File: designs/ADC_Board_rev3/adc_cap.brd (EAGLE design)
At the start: 100 x 80 mm, 35 parts, among them Q1 BSS84, Q2 BSS84, Q3 BSS84, Q4 BSS84

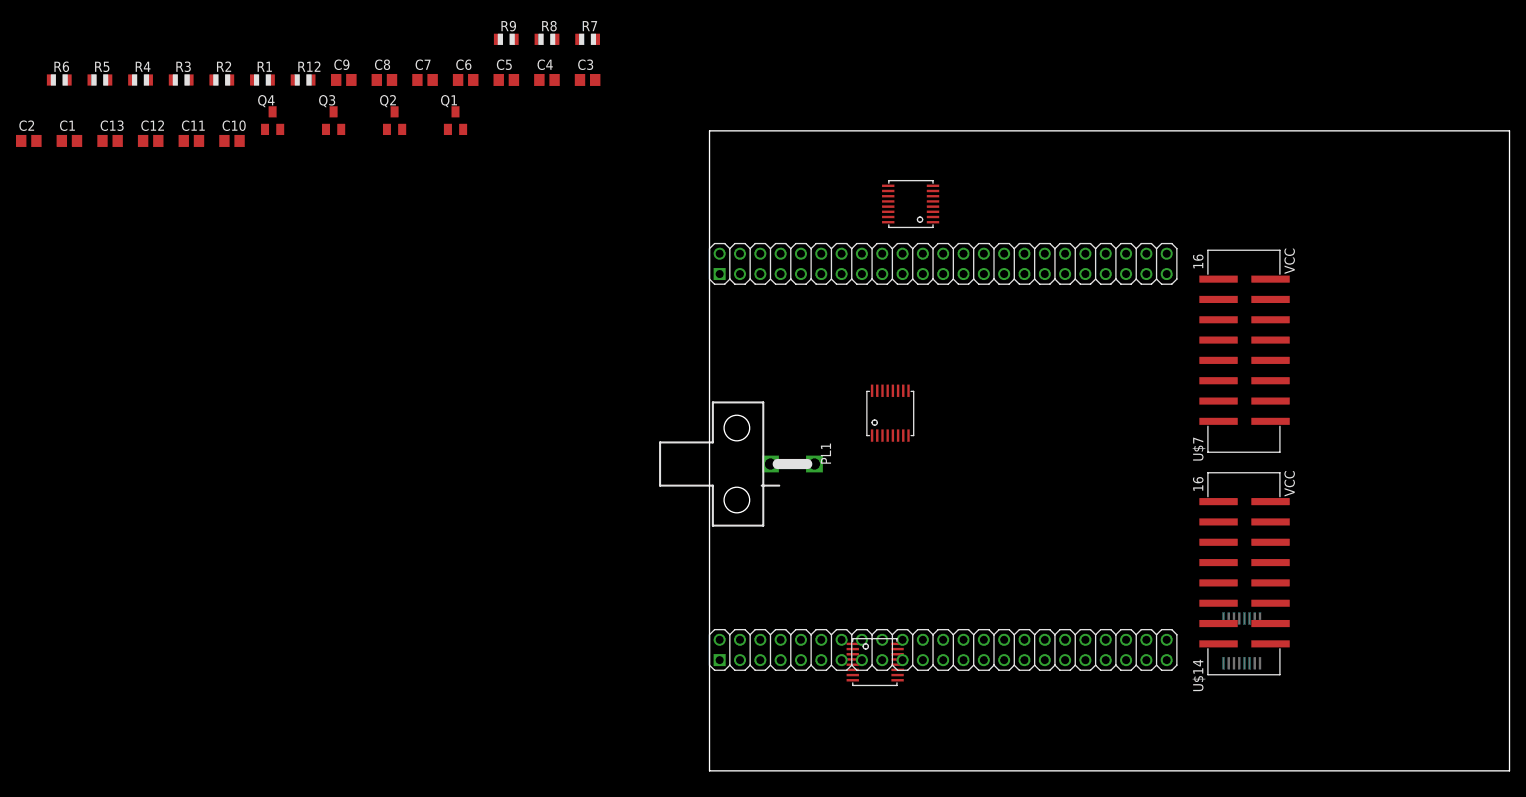
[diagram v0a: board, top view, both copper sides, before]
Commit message: Update on adc rev 3
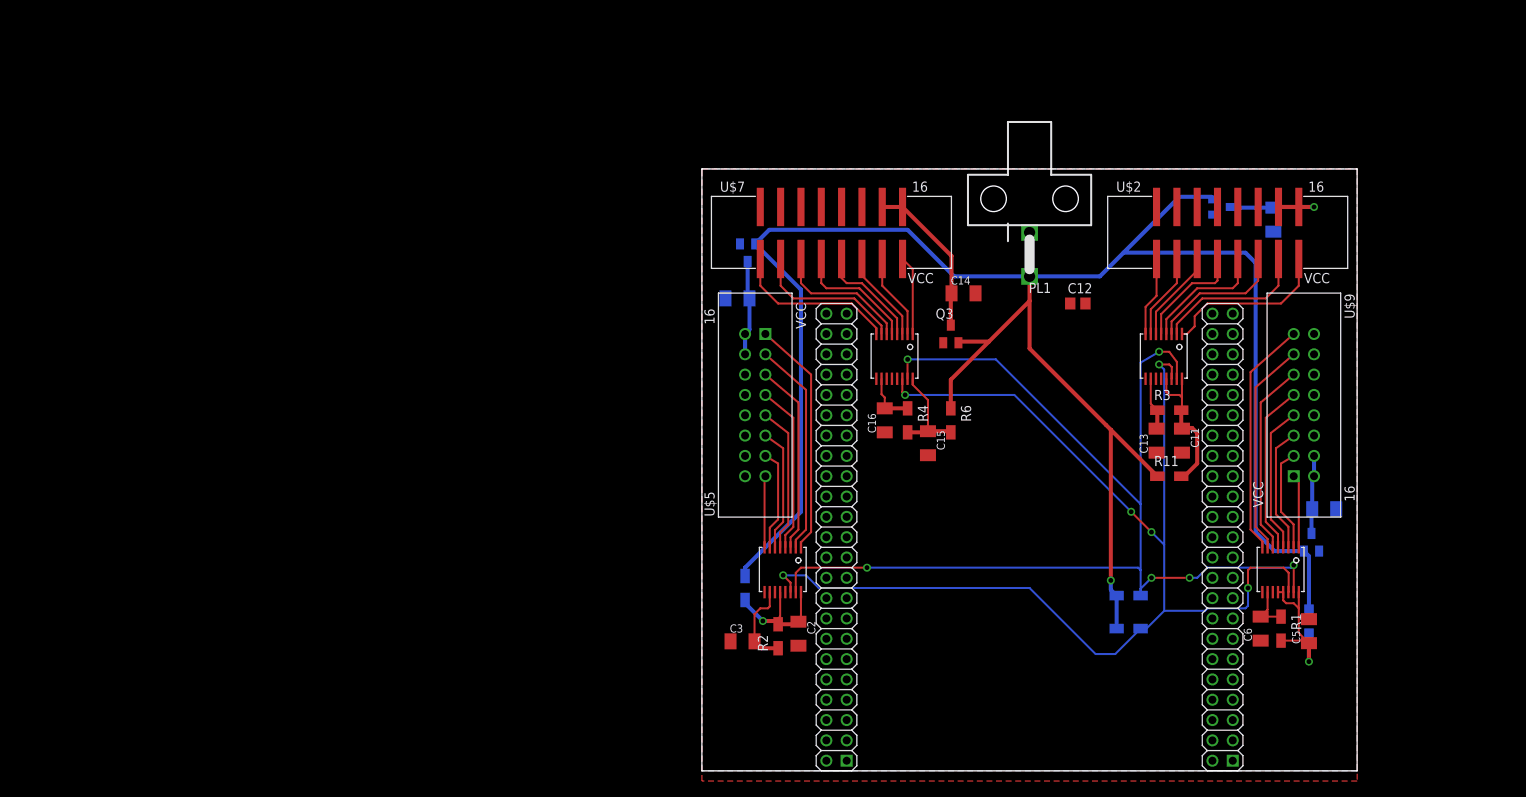
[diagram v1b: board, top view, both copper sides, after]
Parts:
- removed C7, C8, C9: (no value), rcl:C0805
- removed R5, R7, R8: (no value), adafruit:R0805
- removed U$14: 2_X_8_CON, 11_pin_connecterp:2_X_8_PIN
- added C14, C15, C16: (no value), rcl:C1206K
- added R10, R11, R13: (no value), rcl:R1206W
- added U$2: 3020-16-0300-00, TIparts:8X2_SMD_HEADER
- added U$5, U$9: 75869-103LF, TIparts:8X2_THROUGH_HOLE_HEADER
- C1, C10, C11, C13, C2, C3, C4, C5, C6: device rcl:C0805 -> rcl:C1206K
- R1, R12, R2, R3, R4, R6, R9: device adafruit:R0805 -> rcl:R1206W
- U$7: value 2_X_8_CON -> 3020-16-0300-00; device 11_pin_connecterp:2_X_8_PIN -> TIparts:8X2_SMD_HEADER
- moved R1 144.6 mm to (71.4, 17.8), turned to 270 degrees
- moved C13 136.1 mm to (55.9, 41.3), turned to 90 degrees
- moved C10 130.5 mm to (70.5, 68.9), flipped to the bottom, turned to 270 degrees
- moved R3 130.2 mm to (57.5, 45.1)
- moved C11 129.4 mm to (59.1, 41.3), turned to 270 degrees
- moved Q2 126.2 mm to (75.2, 28.6), flipped to the bottom
- moved C5 121.7 mm to (74.9, 17.5), turned to 90 degrees
- moved R12 121.7 mm to (52.4, 21.9), flipped to the bottom, turned to 180 degrees
- moved C6 120.7 mm to (68.9, 17.8), turned to 90 degrees
- moved R6 119.3 mm to (30.2, 43.8), turned to 270 degrees
- moved Q4 119.2 mm to (64.1, 70.5), flipped to the bottom, turned to 90 degrees
- moved C12 117.7 mm to (46.0, 58.4)
- moved C2 114.2 mm to (11.1, 17.1), turned to 270 degrees
- moved C4 111.0 mm to (76.8, 32.7), flipped to the bottom, turned to 180 degrees
- moved R4 104.9 mm to (24.8, 43.8), turned to 270 degrees
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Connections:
- removed net N$11: C1.1, R2.2, U$3.16
- new net N$37: U$7.1, U$8.1
- net GND: now also C13.1, C14.2, C15.2, C16.1, C3.1, C6.1, U$2.10, U$2.11, U$2.12, U$2.13, U$2.14, U$2.9, U$3.11, U$4.11, U$5.10, U$5.11, U$5.12, U$5.13, U$5.14, U$5.9, U$6.11, U$7.10, U$7.11, U$7.12, U$7.13, U$7.14, U$7.9, U$8.11, U$9.10, U$9.11, U$9.12, U$9.13, U$9.14, U$9.9; no longer C13.2, C3.2, C6.2, C7.2, C8.2, C9.2, U$14.3, U$14.4, U$14.5, U$14.6, U$14.7, U$14.8, U$7.3, U$7.4, U$7.5, U$7.6, U$7.7, U$7.8
- net N$1: now also U$2.1; no longer U$14.9
- net N$10: no longer R5.2
- net N$12: now also C13.2, R3.1; no longer C2.1
- net N$13: now also R13.2; no longer R3.2, R7.2, R8.1
- net N$14: now also C1.1, U$5.15, U$5.16; no longer C4.1
- net N$15: now also U$5.1
- net N$16: now also U$5.2
- net N$17: now also U$5.3
- net N$18: now also U$5.4
- net N$19: now also U$5.5
- net N$2: now also R12.2; no longer R1.2, R4.2, R5.1
- net N$20: now also U$5.6
- net N$21: now also U$5.7
- net N$22: now also U$5.8
- net N$23: no longer R4.1
- net N$24: no longer R8.2
- net N$25: now also C11.1, R11.2, R3.2, U$3.13, U$3.16; no longer C5.1, R6.2, U$4.16
- net N$26: now also C3.2, R2.1; no longer C6.1
- net N$27: now also C4.1, U$9.15, U$9.16; no longer C7.1
- net N$28: now also U$9.1
- net N$29: now also U$9.2
- net N$3: now also U$2.2; no longer U$14.10
- net N$30: now also U$9.3
- net N$31: now also U$9.4
- net N$32: now also U$9.5
- net N$33: now also U$9.6
- net N$34: now also U$9.7
- net N$35: now also U$9.8
- net N$36: no longer R7.1
- net N$38: now also C2.1, R2.2, U$4.12, U$4.16; no longer C8.1, U$6.16
- net N$39: now also C6.2, R1.1; no longer C9.1
- net N$4: now also U$2.3; no longer U$14.11
- net N$40: now also C14.1, U$7.15, U$7.16; no longer C10.1, U$7.1, U$7.2
- net N$41: now also U$7.2, U$8.2; no longer U$7.9, U$8.1
- net N$42: now also U$7.3, U$8.3; no longer U$7.10, U$8.2
- net N$43: now also U$7.4, U$8.4; no longer U$7.11, U$8.3
- net N$44: now also U$7.5, U$8.5; no longer U$7.12, U$8.4
- net N$45: now also U$7.6, U$8.6; no longer U$7.13, U$8.5
- net N$46: now also U$7.7, U$8.7; no longer U$7.14, U$8.6
- net N$47: now also U$7.8, U$8.8; no longer U$7.15, U$8.7
- net N$48: now also C5.1, R1.2, R10.2, U$6.12, U$6.13, U$6.16; no longer U$7.16, U$8.8
- net N$5: now also U$2.4; no longer U$14.12
- net N$51: now also C15.1, R4.2, R6.2; no longer C11.1, R12.2
- net N$52: now also C16.2, R4.1; no longer C13.1
- net N$6: now also U$2.5; no longer U$14.13
- net N$7: now also U$2.6; no longer U$14.14
- net N$76: now also C10.1, U$2.15, U$2.16; no longer C3.1, U$14.1, U$14.2
- net N$8: now also U$2.7; no longer U$14.15
- net N$9: now also U$2.8; no longer U$14.16
- net VCC: now also R10.1, R11.1, R13.1; no longer R1.1, R2.1, R3.1, U$3.13, U$4.12, U$6.12, U$6.13
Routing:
- net VCC: track 0.00 -> 255.1 mm, vias 0 -> 1
- net N$13: track 0.00 -> 156.1 mm, vias 0 -> 6
- net N$2: track 0.00 -> 146.3 mm, vias 0 -> 6
- net N$15: track 0.00 -> 29.8 mm
- net N$35: track 0.00 -> 29.7 mm
- net N$16: track 0.00 -> 27.0 mm
- net N$34: track 0.00 -> 26.9 mm
- net N$33: track 0.00 -> 24.1 mm
- net N$17: track 0.00 -> 23.9 mm
- net N$32: track 0.00 -> 21.3 mm
- net N$1: track 0.00 -> 21.2 mm
- net N$18: track 0.00 -> 21.1 mm
- net N$47: track 0.00 -> 20.8 mm
- net N$48: track 0.00 -> 20.1 mm, vias 0 -> 1
- net N$40: track 0.00 -> 19.9 mm
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- added copper zone on layer 1, net GND
- added copper zone on layer 16, net GND
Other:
- board size 100 x 80 mm -> 81.9 x 75.2 mm
